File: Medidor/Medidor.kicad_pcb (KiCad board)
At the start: 2 copper layers, 60 x 47.1 mm, 52 parts, among them J1 TC2030-CTX-TAG_CONECT, SW1 Rotary_Encoder_Switch, SW2 SW_DPST_x2, U1 INA219-INA, U10 spacer, U2 Serial, U3 2450AT18D0100, U4 Fiducial, U5 Fiducial, U6 Fiducial, U7 spacer, U8 spacer, U9 spacer, X1 32MHz

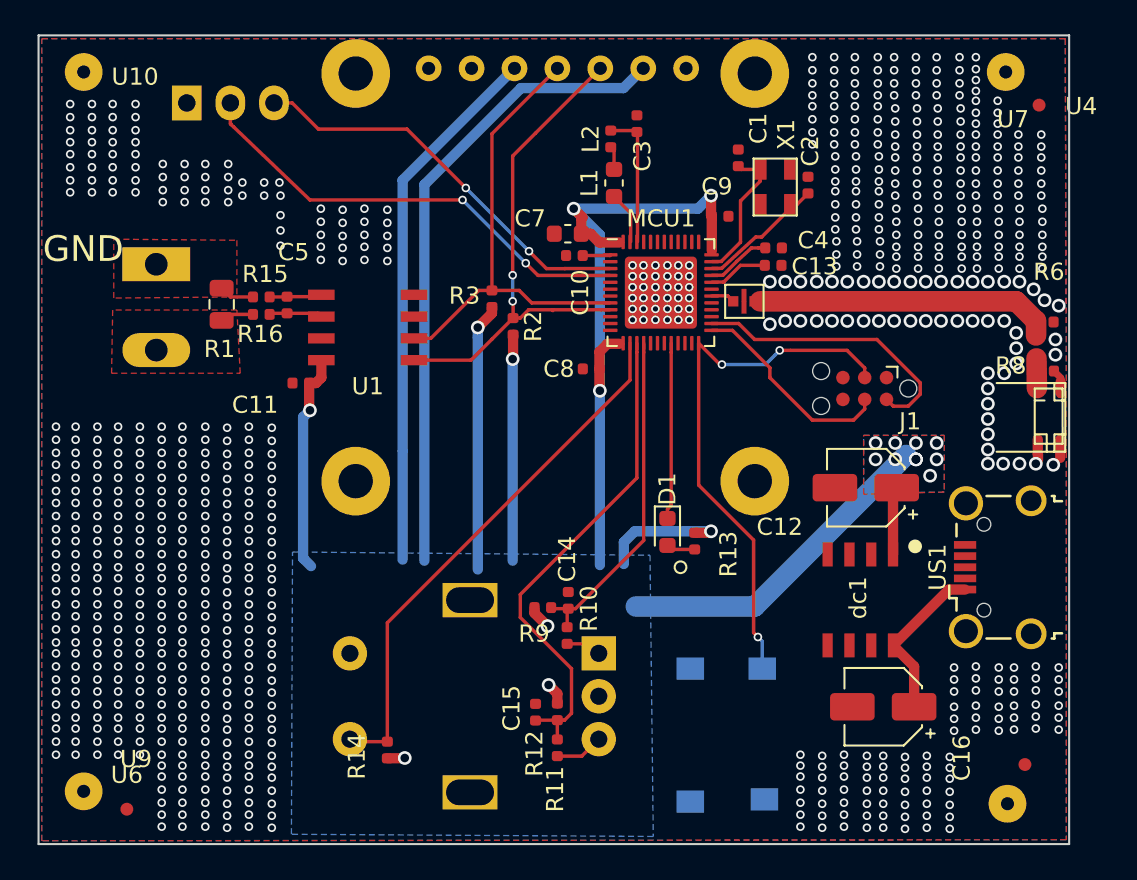
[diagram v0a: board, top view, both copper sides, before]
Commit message: Acabamento
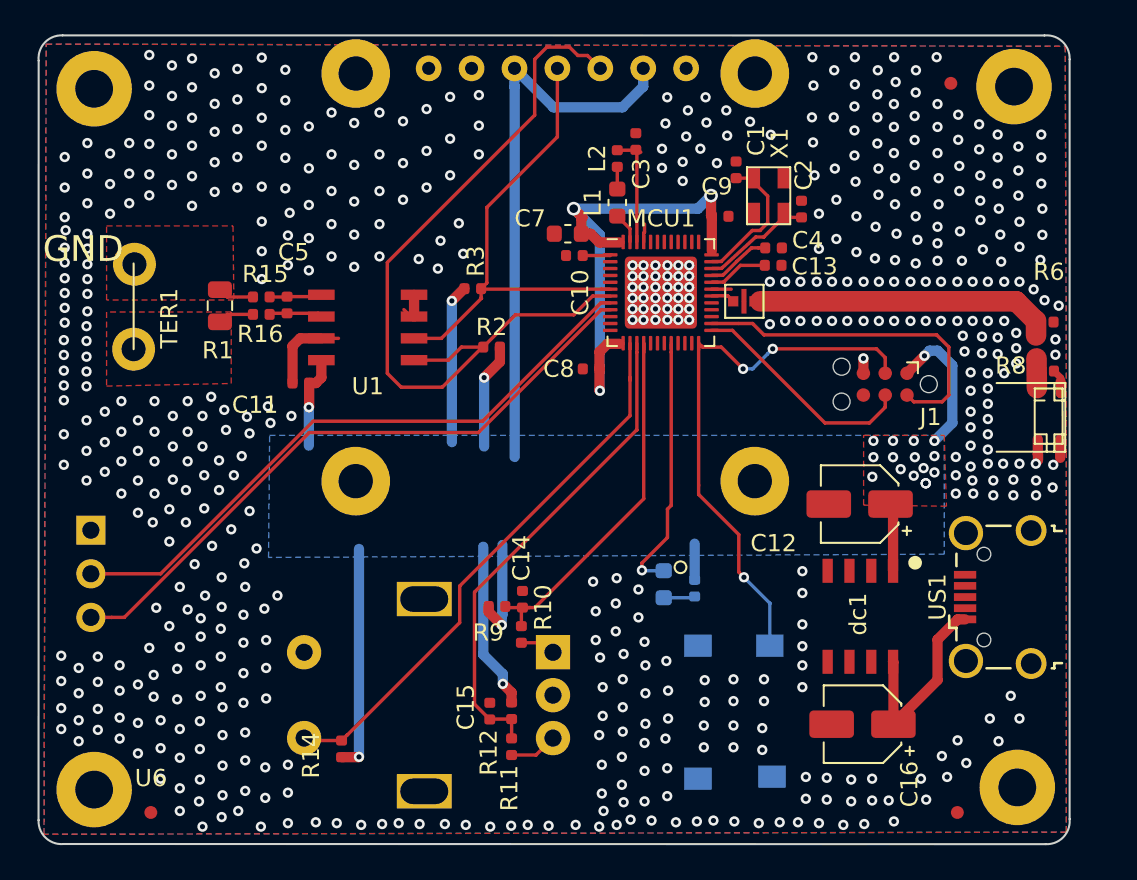
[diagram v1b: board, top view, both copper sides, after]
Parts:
- removed Screw_Terminal: TerminalBlock_Altech_AK300-2_P5.00mm, TerminalBlock:TerminalBlock_Altech_AK300-2_P5.00mm
- removed U10, U7, U8, U9: spacer, Medidor:spacer
- added G***: LOGO, Medidor:multi1, F.Cu at (141.7, 99.9)
- added REF**: MountingHole_2.2mm_M2_Pad, MountingHole:MountingHole_2.2mm_M2_Pad, F.Cu at (140.6, 132.1)
- added REF**: MountingHole_2.2mm_M2_Pad, MountingHole:MountingHole_2.2mm_M2_Pad, F.Cu at (140.4, 91.2)
- added REF**: MountingHole_2.2mm_M2_Pad, MountingHole:MountingHole_2.2mm_M2_Pad, F.Cu at (86.8, 132.2)
- added REF**: MountingHole_2.2mm_M2_Pad, MountingHole:MountingHole_2.2mm_M2_Pad, F.Cu at (86.8, 91.4)
- added TER1: terminal-medidor, Medidor:Screw, F.Cu at (89.1, 101.5)
- D1, R13: moved to B.Cu
- U2: footprint Connector:FanPinHeader_1x03_P2.54mm_Vertical -> Connector_PinHeader_2.54mm:PinHeader_1x03_P2.54mm_Vertical
- moved U2 25.5 mm to (86.6, 117.1), turned to 180 degrees
- moved U4 5.30 mm to (136.7, 91.1)
- moved U5 4.83 mm to (137.1, 133.5)
- moved D1 3.06 mm to (120.0, 120.2)
- moved R13 2.74 mm to (121.8, 120.5)
- moved C14 2.67 mm to (111.8, 121.1)
- moved C15 2.67 mm to (109.9, 127.6)
- moved R10 2.67 mm to (111.7, 123.2)
- moved R12 2.67 mm to (111.1, 127.6)
- moved R14 2.67 mm to (101.2, 129.8)
- moved R9 2.67 mm to (110.3, 121.5)
- moved SW1 2.67 mm to (113.5, 124.2)
- moved R11 2.67 mm to (111.1, 129.7)
- moved R2 1.74 mm to (110.0, 106.4), turned to 0 degrees
- moved US1 1.74 mm to (139.4, 121.0)
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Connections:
- MCU1 pad 3: /TX -> Net-(MCU1-Pad3)
- MCU1 pad 4: /RX -> Net-(MCU1-Pad4)
- MCU1 pad 6: Net-(MCU1-Pad6) -> SDA
- MCU1 pad 7: Net-(MCU1-Pad7) -> SCL
- MCU1 pad 8: SDA -> /RX
- MCU1 pad 9: SCL -> /TX
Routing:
- net +3V3: track 185.8 -> 127.3 mm, vias 20 -> 25
- net SCL: track 29.4 -> 46.2 mm, vias 2 -> 0
- net /TX: track 23.6 -> 37.7 mm, vias 2 -> 0
- net GND: track 3.76 -> 13.9 mm, vias 783 -> 558
- net /RX: track 26.9 -> 36.8 mm, vias 2 -> 0
- net LEDMCU: track 10.3 -> 15.2 mm, vias 0 -> 1
- net SWDIO: track 16.7 -> 20.0 mm
- net RC1: track 19.7 -> 21.8 mm
- net +5V: track 9.63 -> 11.7 mm
- net Net-(L1-Pad1): track 3.04 -> 1.81 mm
- net SWDCLK: track 12.3 -> 13.4 mm
- net RC3: track 31.3 -> 32.5 mm
- net Net-(C3-Pad2): track 7.87 -> 6.94 mm
- net Net-(C2-Pad2): track 7.48 -> 6.73 mm
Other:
- board size 60 x 47.1 mm -> 60.1 x 47.1 mm
- net class Ant: via_dia 0.5 -> 0.6
- net class Default: via_dia 0.5 -> 0.6
- net class Suply: via_dia 0.8 -> 0.6; via_drill 0.5 -> 0.3
- board text added: "Meter One for All UFAL C.I. 2019.1 José Carlos Pinheiro Filho Glauber Braga Tatiane"
